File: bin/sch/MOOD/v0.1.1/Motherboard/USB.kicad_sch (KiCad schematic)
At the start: 11 parts

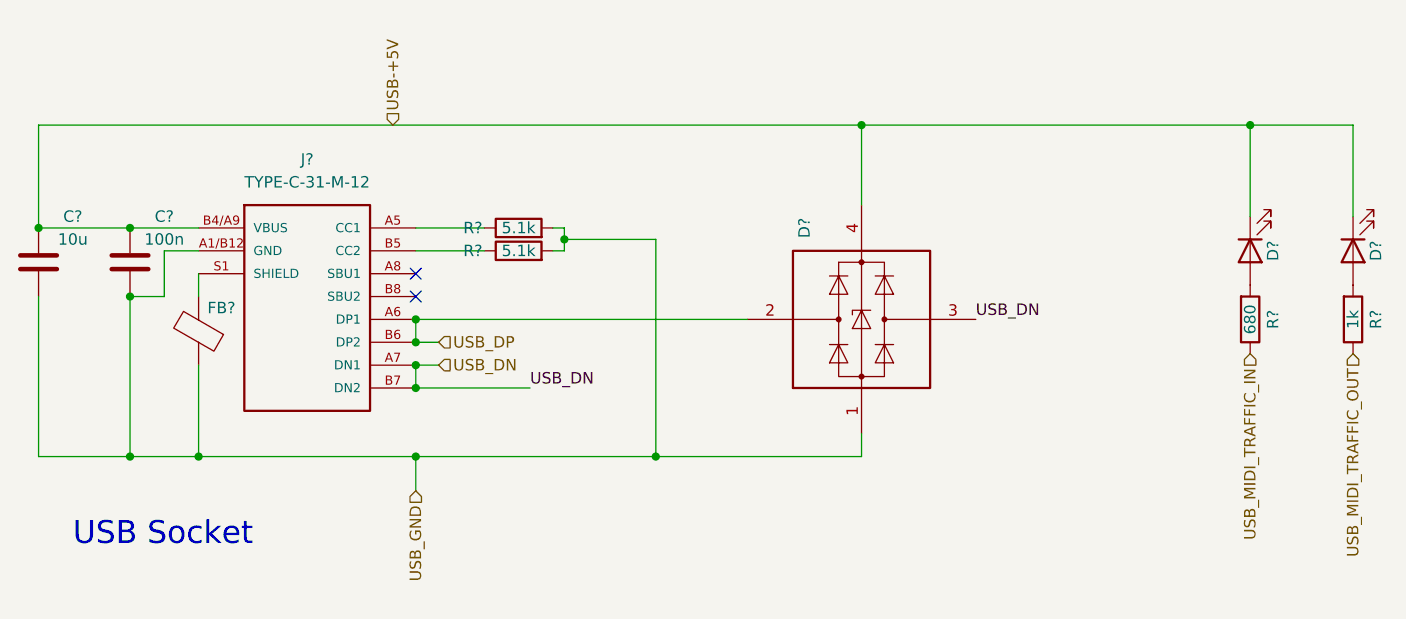
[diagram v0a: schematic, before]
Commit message: -	Made a bunch of changes -	Added KeyboardCard
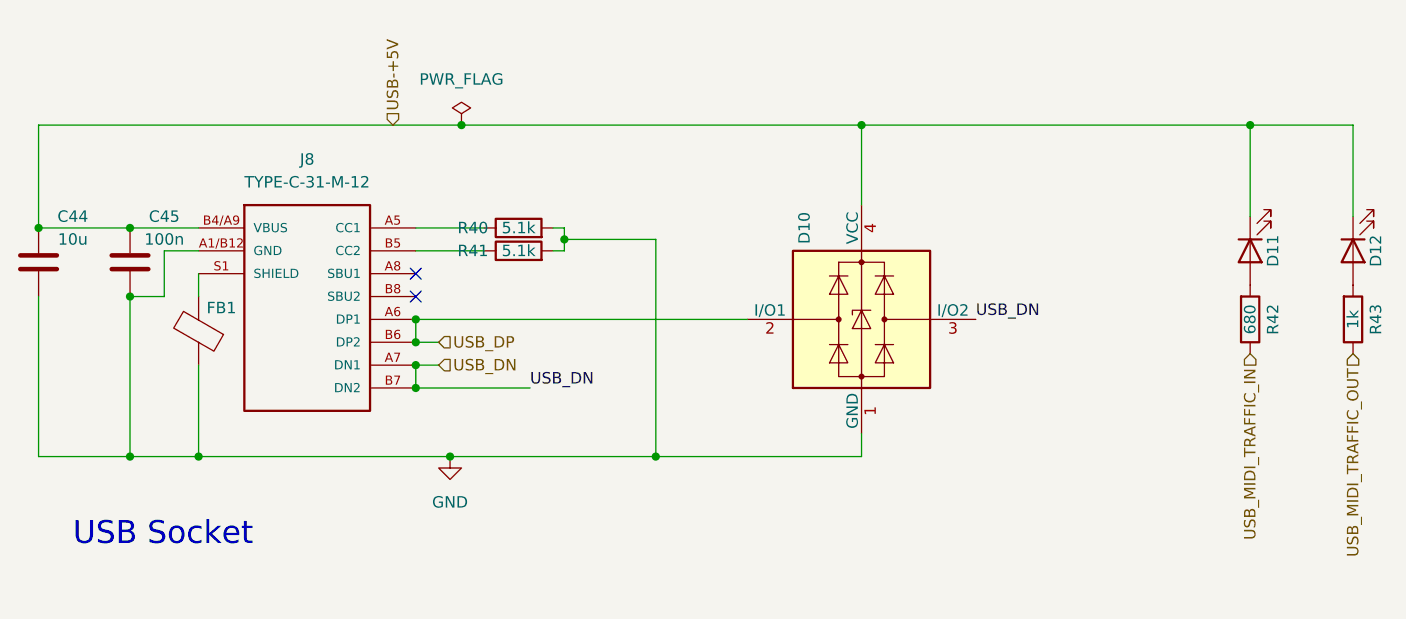
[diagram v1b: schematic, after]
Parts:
- gave numbers to parts that had none: 11
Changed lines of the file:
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@@
   (junction (at 83.82 55.88) (diameter 0) (color 0 0 0 0)
   )
+  (junction (at 88.9 31.75) (diameter 0) (color 0 0 0 0)
+  )
   (junction (at 83.82 60.96) (diameter 0) (color 0 0 0 0)
   )
@@
   (junction (at 133.35 31.75) (diameter 0) (color 0 0 0 0)
   )
-  (junction (at 83.82 68.58) (diameter 0) (color 0 0 0 0)
-  )
   (junction (at 52.07 50.8) (diameter 0) (color 0 0 0 0)
   )
   (junction (at 52.07 43.18) (diameter 0) (color 0 0 0 0)
+  )
+  (junction (at 87.63 68.58) (diameter 0) (color 0 0 0 0)
   )
   (junction (at 100.33 44.45) (diameter 0) (color 0 0 0 0)
@@
     (stroke (width 0) (type default) (color 0 0 0 0))
   )
-  (wire (pts (xy 83.82 72.39) (xy 83.82 68.58))
-    (stroke (width 0) (type default) (color 0 0 0 0))
-  )
-  (wire (pts (xy 83.82 68.58) (xy 59.69 68.58))
+  (wire (pts (xy 59.69 68.58) (xy 87.63 68.58))
     (stroke (width 0) (type default) (color 0 0 0 0))
   )
@@
     (stroke (width 0) (type default) (color 0 0 0 0))
   )
+  (wire (pts (xy 87.63 68.58) (xy 110.49 68.58))
+    (stroke (width 0) (type default) (color 0 0 0 0))
+  )
   (wire (pts (xy 176.53 31.75) (xy 176.53 41.91))
     (stroke (width 0) (type default) (color 0 0 0 0))
@@
     (stroke (width 0) (type default) (color 0 0 0 0))
   )
-  (wire (pts (xy 83.82 68.58) (xy 110.49 68.58))
-    (stroke (width 0) (type default) (color 0 0 0 0))
-  )
   (wire (pts (xy 83.82 60.96) (xy 96.52 60.96))
     (stroke (width 0) (type default) (color 0 0 0 0))
   )
+  (wire (pts (xy 88.9 31.75) (xy 133.35 31.75))
+    (stroke (width 0) (type default) (color 0 0 0 0))
+  )
   (wire (pts (xy 99.06 45.72) (xy 100.33 45.72))
     (stroke (width 0) (type default) (color 0 0 0 0))
@@
     (stroke (width 0) (type default) (color 0 0 0 0))
   )
-  (wire (pts (xy 41.91 31.75) (xy 133.35 31.75))
+  (wire (pts (xy 41.91 31.75) (xy 88.9 31.75))
     (stroke (width 0) (type default) (color 0 0 0 0))
   )
@@
     (effects (font (size 1.27 1.27)) (justify right))
   )
-  (hierarchical_label "USB_GND" (shape input) (at 83.82 72.39 270)
-    (effects (font (size 1.27 1.27)) (justify right))
-  )
   (hierarchical_label "USB_DN" (shape input) (at 86.36 58.42 0)
     (effects (font (size 1.27 1.27)) (justify left))
   )
+  (symbol (lib_id "power:PWR_FLAG") (at 88.9 31.75 0) (unit 1)
+    (in_bom yes) (on_board yes) (fields_autoplaced)
+    (property "Reference" "#FLG02" (id 0) (at 88.9 29.845 0)
+      (effects (font (size 1.27 1.27)) hide)
+    )
+    (property "Value" "PWR_FLAG" (id 1) (at 88.9 26.67 0))
+    (property "Footprint" "" (id 2) (at 88.9 31.75 0)
+      (effects (font (size 1.27 1.27)) hide)
+    )
+    (property "Datasheet" "~" (id 3) (at 88.9 31.75 0)
+      (effects (font (size 1.27 1.27)) hide)
+    )
+    (pin "1")
+  )
   (symbol (lib_id "Device:C") (at 52.07 46.99 180) (unit 1)
     (in_bom yes) (on_board yes)
-    (property "Reference" "C?" (id 0) (at 55.88 41.91 0))
+    (property "Reference" "C45" (id 0) (at 55.88 41.91 0))
     (property "Value" "100n" (id 1) (at 55.88 44.45 0))
     (property "Footprint" "Capacitor_SMD:C_0402_1005Metric" (id 2) (at 51.1048 43.18 0)
@@
   (symbol (lib_id "Igor:TYPE-C-31-M-12") (at 64.77 63.5 0) (unit 1)
     (in_bom yes) (on_board yes) (fields_autoplaced)
-    (property "Reference" "J?" (id 0) (at 71.755 35.56 0))
+    (property "Reference" "J8" (id 0) (at 71.755 35.56 0))
     (property "Value" "TYPE-C-31-M-12" (id 1) (at 71.755 38.1 0))
     (property "Footprint" "Igor:TYPE-C-31-M-12" (id 2) (at 54.61 72.39 0)
@@
   (symbol (lib_id "Power_Protection:PRTR5V0U2X") (at 133.35 53.34 0) (unit 1)
     (in_bom yes) (on_board yes)
-    (property "Reference" "D?" (id 0) (at 127 43.18 90))
+    (property "Reference" "D10" (id 0) (at 127 43.18 90))
     (property "Value" "PRTR5V0U2X" (id 1) (at 118.11 41.91 0)
       (effects (font (size 1.27 1.27)) hide)
@@
   (symbol (lib_id "Device:R") (at 95.25 45.72 90) (unit 1)
     (in_bom yes) (on_board yes)
-    (property "Reference" "R?" (id 0) (at 90.17 45.72 90))
+    (property "Reference" "R41" (id 0) (at 90.17 45.72 90))
     (property "Value" "5.1k" (id 1) (at 95.25 45.72 90))
     (property "Footprint" "Resistor_SMD:R_0402_1005Metric" (id 2) (at 95.25 47.498 90)
@@
   (symbol (lib_id "Device:R") (at 95.25 43.18 90) (unit 1)
     (in_bom yes) (on_board yes)
-    (property "Reference" "R?" (id 0) (at 90.17 43.18 90))
+    (property "Reference" "R40" (id 0) (at 90.17 43.18 90))
     (property "Value" "5.1k" (id 1) (at 95.25 43.18 90))
     (property "Footprint" "Resistor_SMD:R_0402_1005Metric" (id 2) (at 95.25 44.958 90)
@@
   (symbol (lib_id "Device:C") (at 41.91 46.99 180) (unit 1)
     (in_bom yes) (on_board yes)
-    (property "Reference" "C?" (id 0) (at 45.72 41.91 0))
+    (property "Reference" "C44" (id 0) (at 45.72 41.91 0))
     (property "Value" "10u" (id 1) (at 45.72 44.45 0))
     (property "Footprint" "Capacitor_SMD:C_0402_1005Metric" (id 2) (at 40.9448 43.18 0)
@@
   (symbol (lib_id "Device:FerriteBead") (at 59.69 54.61 180) (unit 1)
     (in_bom yes) (on_board yes)
-    (property "Reference" "FB?" (id 0) (at 62.23 52.07 0))
+    (property "Reference" "FB1" (id 0) (at 62.23 52.07 0))
     (property "Value" "FerriteBead" (id 1) (at 54.61 54.6608 90)
       (effects (font (size 1.27 1.27)) hide)
@@
   (symbol (lib_id "Device:R") (at 176.53 53.34 0) (mirror x) (unit 1)
     (in_bom yes) (on_board yes)
-    (property "Reference" "R?" (id 0) (at 179.07 53.34 90))
+    (property "Reference" "R42" (id 0) (at 179.07 53.34 90))
     (property "Value" "680" (id 1) (at 176.53 53.34 90))
     (property "Footprint" "Resistor_SMD:R_0402_1005Metric" (id 2) (at 174.752 53.34 90)
@@
     (pin "2")
   )
+  (symbol (lib_id "power:GND") (at 87.63 68.58 0) (unit 1)
+    (in_bom yes) (on_board yes) (fields_autoplaced)
+    (property "Reference" "#PWR0107" (id 0) (at 87.63 74.93 0)
+      (effects (font (size 1.27 1.27)) hide)
+    )
+    (property "Value" "GND" (id 1) (at 87.63 73.66 0))
+    (property "Footprint" "" (id 2) (at 87.63 68.58 0)
+      (effects (font (size 1.27 1.27)) hide)
+    )
+    (property "Datasheet" "" (id 3) (at 87.63 68.58 0)
+      (effects (font (size 1.27 1.27)) hide)
+    )
+    (pin "1")
+  )
   (symbol (lib_id "Device:R") (at 187.96 53.34 0) (mirror x) (unit 1)
     (in_bom yes) (on_board yes)
-    (property "Reference" "R?" (id 0) (at 190.5 53.34 90))
+    (property "Reference" "R43" (id 0) (at 190.5 53.34 90))
     (property "Value" "1k" (id 1) (at 187.96 53.34 90))
     (property "Footprint" "Resistor_SMD:R_0402_1005Metric" (id 2) (at 186.182 53.34 90)
@@
   (symbol (lib_id "Device:LED") (at 176.53 45.72 90) (mirror x) (unit 1)
     (in_bom yes) (on_board yes)
-    (property "Reference" "D?" (id 0) (at 179.07 45.72 0))
+    (property "Reference" "D11" (id 0) (at 179.07 45.72 0))
     (property "Value" "Green" (id 1) (at 181.61 44.1325 0)
       (effects (font (size 1.27 1.27)) hide)
@@
   (symbol (lib_id "Device:LED") (at 187.96 45.72 90) (mirror x) (unit 1)
     (in_bom yes) (on_board yes)
-    (property "Reference" "D?" (id 0) (at 190.5 45.72 0))
+    (property "Reference" "D12" (id 0) (at 190.5 45.72 0))
     (property "Value" "Blue" (id 1) (at 193.04 44.1325 0)
       (effects (font (size 1.27 1.27)) hide)
